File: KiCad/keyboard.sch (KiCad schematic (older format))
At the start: 130 parts

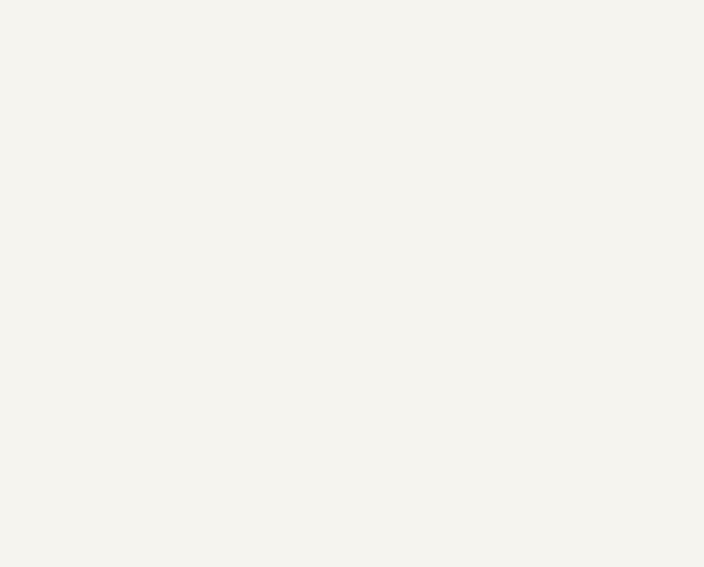
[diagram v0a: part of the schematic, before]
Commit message: Wired USB
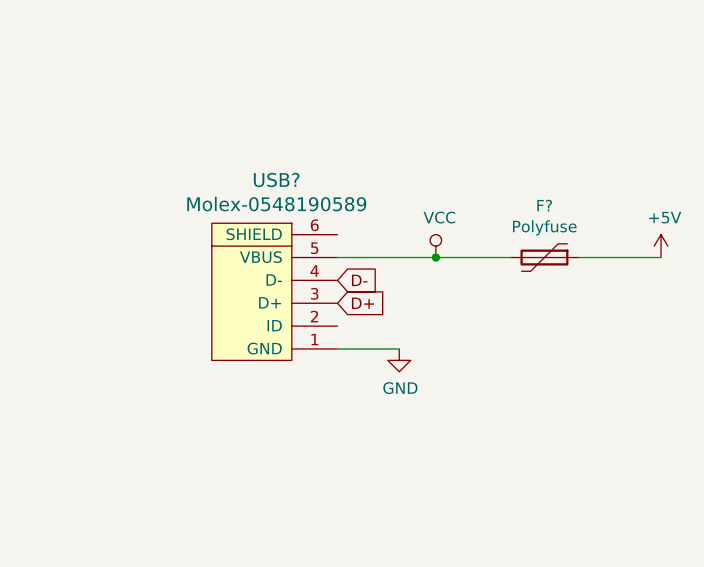
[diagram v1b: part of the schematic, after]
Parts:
- added F?: Polyfuse, symbol Device:Polyfuse
- added USB?: Molex-0548190589, symbol random-keyboard-parts:Molex-0548190589
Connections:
- net +5V: now also F?.1
- net D+: now also USB?.3 (D+)
- net D-: now also USB?.4 (D-)
- net GND: now also USB?.1 (GND)
- new net VCC: F?.2, USB?.5 (VBUS)
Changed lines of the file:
@@
 Text GLabel 11535 10035 0    50   Input ~ 0
 D-
+$Comp
+L random-keyboard-parts:Molex-0548190589 USB?
+U 1 1 6149CA0B
+P 17820 6560
+F 0 "USB?" V 18357 6527 60  0000 C CNN
+F 1 "Molex-0548190589" V 18251 6527 60  0000 C CNN
+F 2 "" H 17820 6560 60  0001 C CNN
+F 3 "" H 17820 6560 60  0001 C CNN
+	1    17820 6560
+	0    -1   -1   0
+$EndComp
+$Comp
+L power:VCC #PWR?
+U 1 1 614EF491
+P 18550 6360
+F 0 "#PWR?" H 18550 6210 50  0001 C CNN
+F 1 "VCC" H 18567 6533 50  0000 C CNN
+F 2 "" H 18550 6360 50  0001 C CNN
+F 3 "" H 18550 6360 50  0001 C CNN
+	1    18550 6360
+	1    0    0    -1
+$EndComp
+$Comp
+L Device:Polyfuse F?
+U 1 1 614F0170
+P 19025 6360
+F 0 "F?" V 18800 6360 50  0000 C CNN
+F 1 "Polyfuse" V 18891 6360 50  0000 C CNN
+F 2 "" H 19075 6160 50  0001 L CNN
+F 3 "~" H 19025 6360 50  0001 C CNN
+	1    19025 6360
+	0    1    1    0
+$EndComp
+$Comp
+L power:+5V #PWR?
+U 1 1 614F0D68
+P 19535 6360
+F 0 "#PWR?" H 19535 6210 50  0001 C CNN
+F 1 "+5V" H 19550 6533 50  0000 C CNN
+F 2 "" H 19535 6360 50  0001 C CNN
+F 3 "" H 19535 6360 50  0001 C CNN
+	1    19535 6360
+	1    0    0    -1
+$EndComp
+Wire Wire Line
+	18120 6360 18550 6360
+Wire Wire Line
+	18550 6360 18875 6360
+Connection ~ 18550 6360
+Wire Wire Line
+	19175 6360 19535 6360
+$Comp
+L power:GND #PWR?
+U 1 1 61530793
+P 18390 6760
+F 0 "#PWR?" H 18390 6510 50  0001 C CNN
+F 1 "GND" H 18395 6587 50  0000 C CNN
+F 2 "" H 18390 6760 50  0001 C CNN
+F 3 "" H 18390 6760 50  0001 C CNN
+	1    18390 6760
+	1    0    0    -1
+$EndComp
+Wire Wire Line
+	18390 6760 18120 6760
+Text GLabel 18120 6460 2    50   Input ~ 0
+D-
+Text GLabel 18120 6560 2    50   Input ~ 0
+D+
 $EndSCHEMATC
